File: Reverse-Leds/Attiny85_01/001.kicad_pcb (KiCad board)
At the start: 2 copper layers, 10.2 x 10.2 mm, 4 parts, among them IC1 ATTINY85-20SU, J1 Conn_01x04, J2 Conn_01x04, U2 Firma

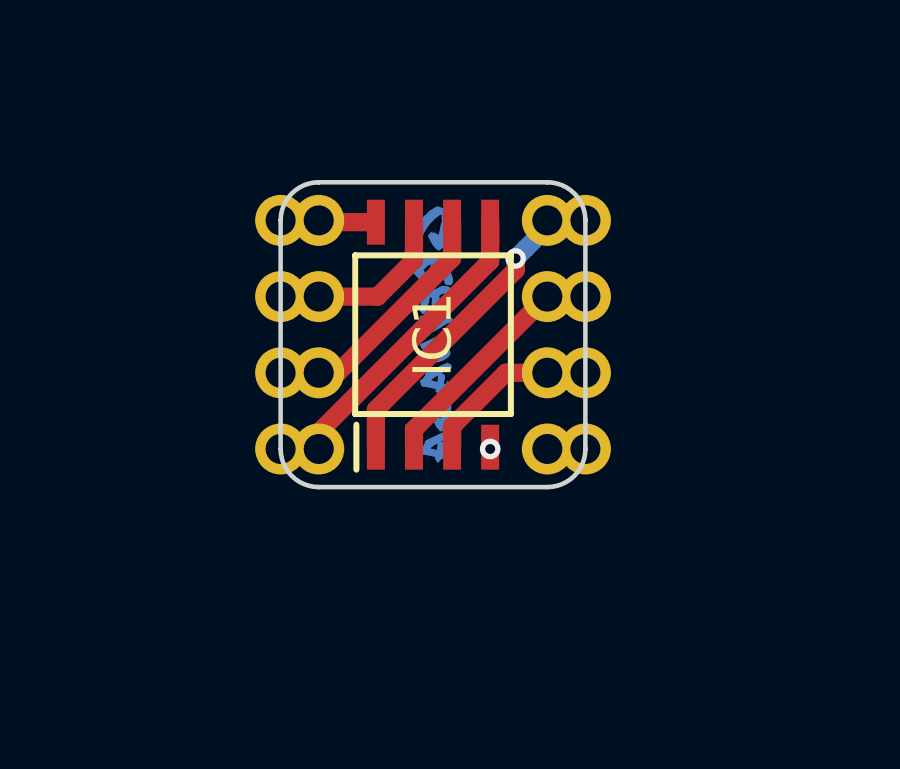
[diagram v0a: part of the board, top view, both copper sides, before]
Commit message: Add Heart Logo
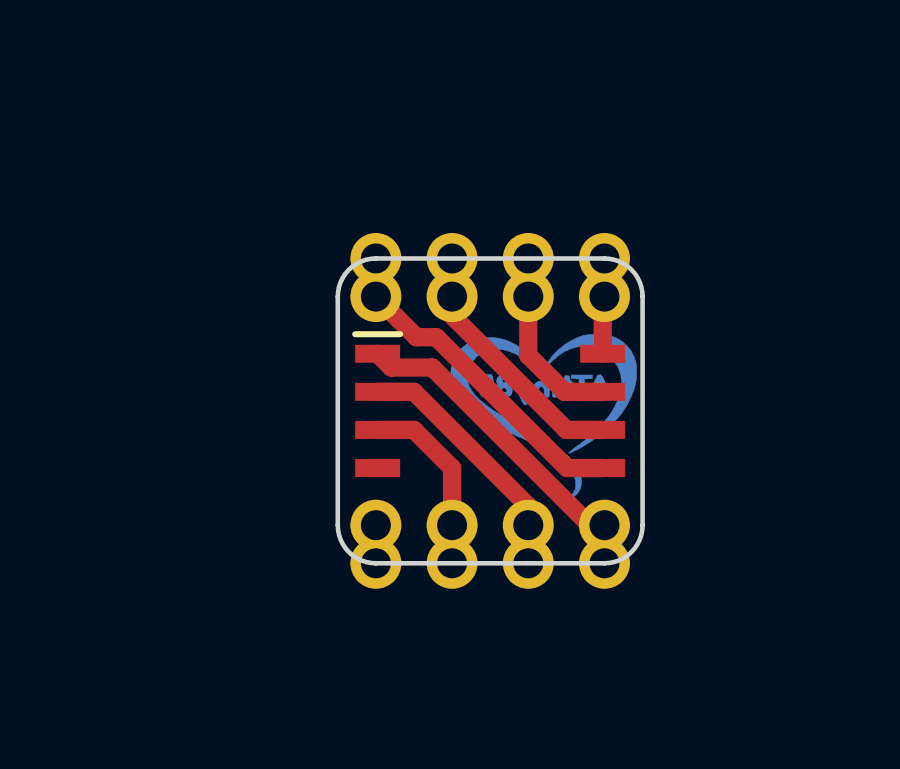
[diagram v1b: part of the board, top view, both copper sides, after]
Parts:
- removed U2: Firma, Charly_Plex_6_Leds_Ala_Gaviota_Moon_75mm:firma_Cu_Mask
- added Ref**: Val**, Attiny85_01:Firma_New, F.Cu at (145.8, 99.6)
- added Ref**: Val**, Attiny85_01:Heart, F.Cu at (150.1, 99.9)
- J1: footprint Attiny85:Attiny85_Socket_Castell_Up -> Attiny85_01:Attiny85_Socket_Castell_Up
- J2: footprint Attiny85:Attiny85_Socket_Castell_Down -> Attiny85_01:Attiny85_Socket_Castell_Down
- moved J2 10.3 mm to (153.7, 103.5), turned to 270 degrees
- moved J1 5.43 mm to (146.1, 95.9), turned to 90 degrees
- moved IC1 3.17 mm to (149.9, 99.7), turned to 0 degrees
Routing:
- net Net-(IC1-Pad1): vias 1 -> 0
- net GND: vias 1 -> 0
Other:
- board text added: "Developed by"
